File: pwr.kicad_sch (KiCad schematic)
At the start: 2 parts, among them J2 ATX-24, J3 Conn_02x02_Top_Bottom

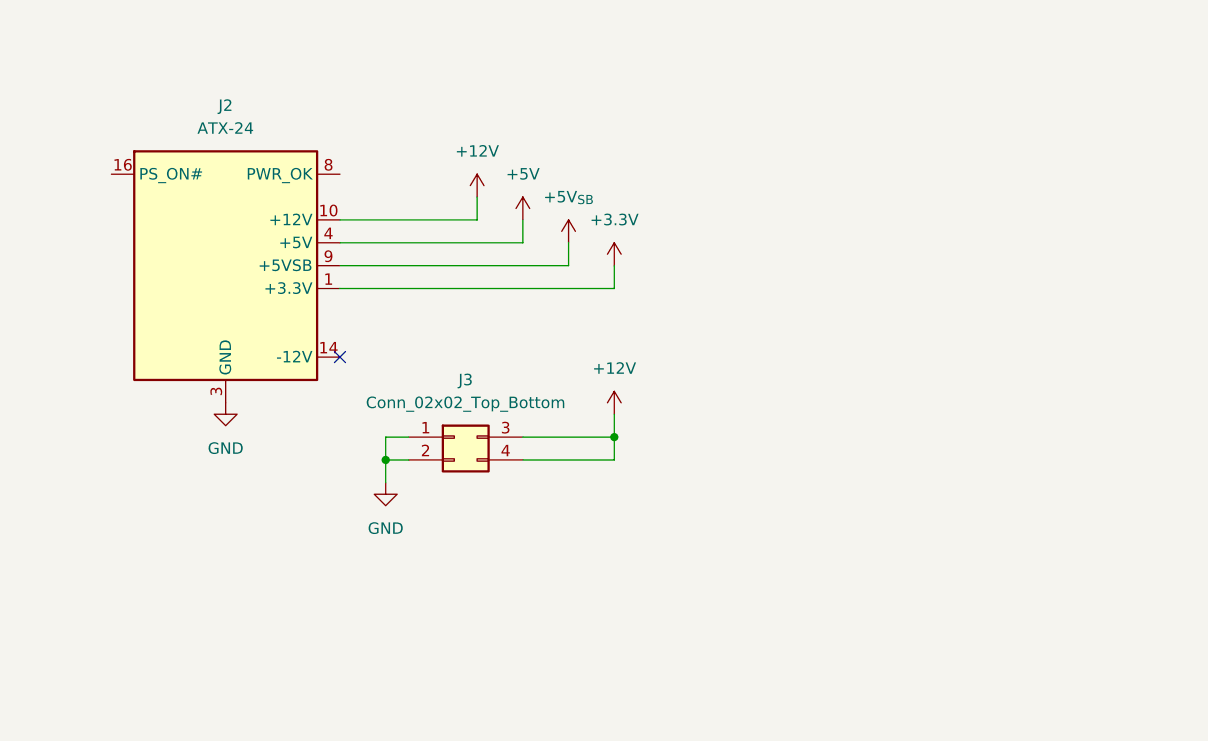
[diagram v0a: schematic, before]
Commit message: Cleanup & Debug I/O
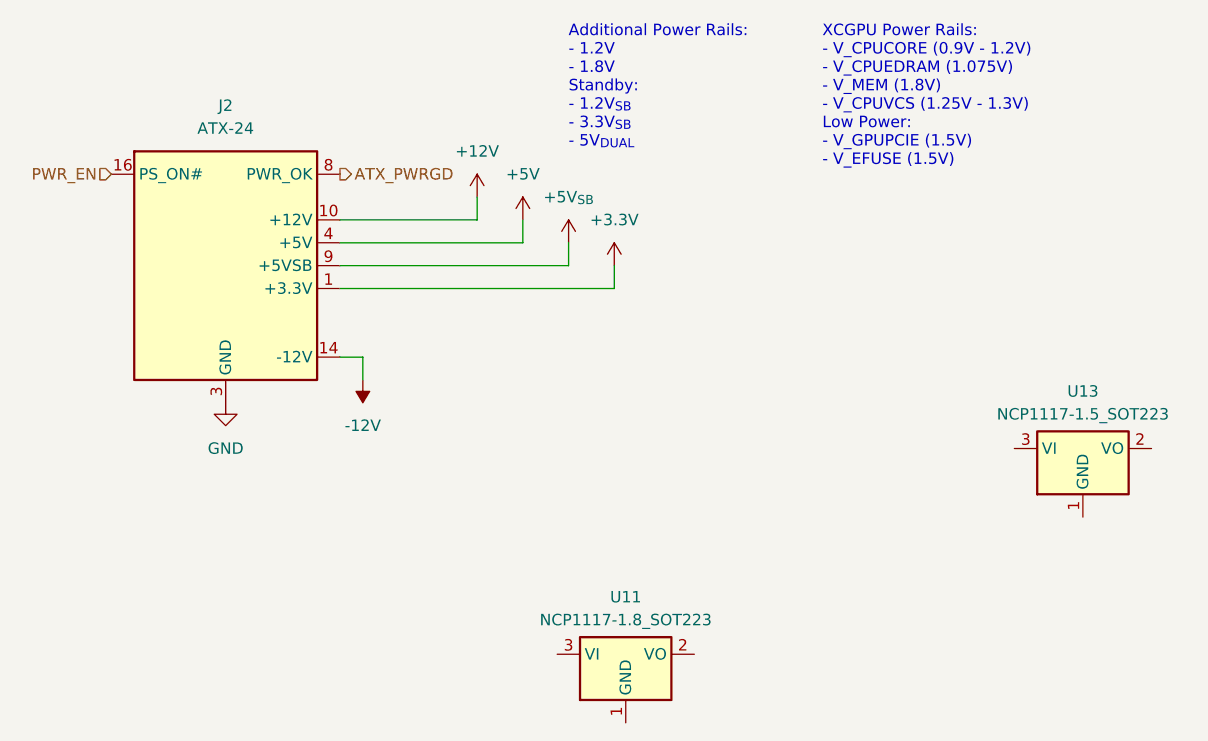
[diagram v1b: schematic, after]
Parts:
- removed J3: Conn_02x02_Top_Bottom, symbol Connector_Generic:Conn_02x02_Top_Bottom
- added U11: NCP1117-1.8_SOT223, Package_TO_SOT_SMD:SOT-223-3_TabPin2, symbol Regulator_Linear:NCP1117-1.8_SOT223
- added U13: NCP1117-1.5_SOT223, Package_TO_SOT_SMD:SOT-223-3_TabPin2, symbol Regulator_Linear:NCP1117-1.5_SOT223
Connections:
- net -12V: now reaches J2.14 (-12V)
- net PWR_EN: now reaches J2.16 (PS_ON#)
- net ATX_PWRGD: now reaches J2.8 (PWR_OK)
- no-connect marks 1 -> 0
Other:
- note added: "Additional Power Rails: - 1.2V - 1.8V Standby: - 1.2V_{SB} - 3.3V_{SB} - 5V_{DUAL}"
- note added: "XCGPU Power Rails: - V_CPUCORE (0.9V - 1.2V) - V_CPUEDRAM (1.075V) - V_MEM (1.8V) - V_CPUVCS (1.25V - 1.3V) Low Power: - V_GPUPCIE (1.5V) - V_EFUSE (1.5V)"
